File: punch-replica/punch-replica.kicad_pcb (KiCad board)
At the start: 2 copper layers, 90 x 80 mm, 67 parts, among them J10 Screw_Terminal_01x03, J11 Screw_Terminal_01x03, J12 Screw_Terminal_01x02, J2 12V PSU, J3 5V OUT, J4 5V OUT, J5 LOAD CELL, J6 COIN SLOT, J7 Conn_01x02_Socket, J9 IDC_Connector, K1 SRD-05VDC-SL-C, K2 SRD-05VDC-SL-C, Q1 BSS138, Q2 BSS138, Q3 Q_NMOS_Depletion_GSD, Q4 Q_NMOS_Depletion_GSD, SW1 SW_Push, SW2 SW_Push, U1 LM2596S-5, U2 AMS1117-3.3, U3 CH340C, U4 PC817, U5 PC817, U6 ESP32-WROOM-32, U7 DFR0299

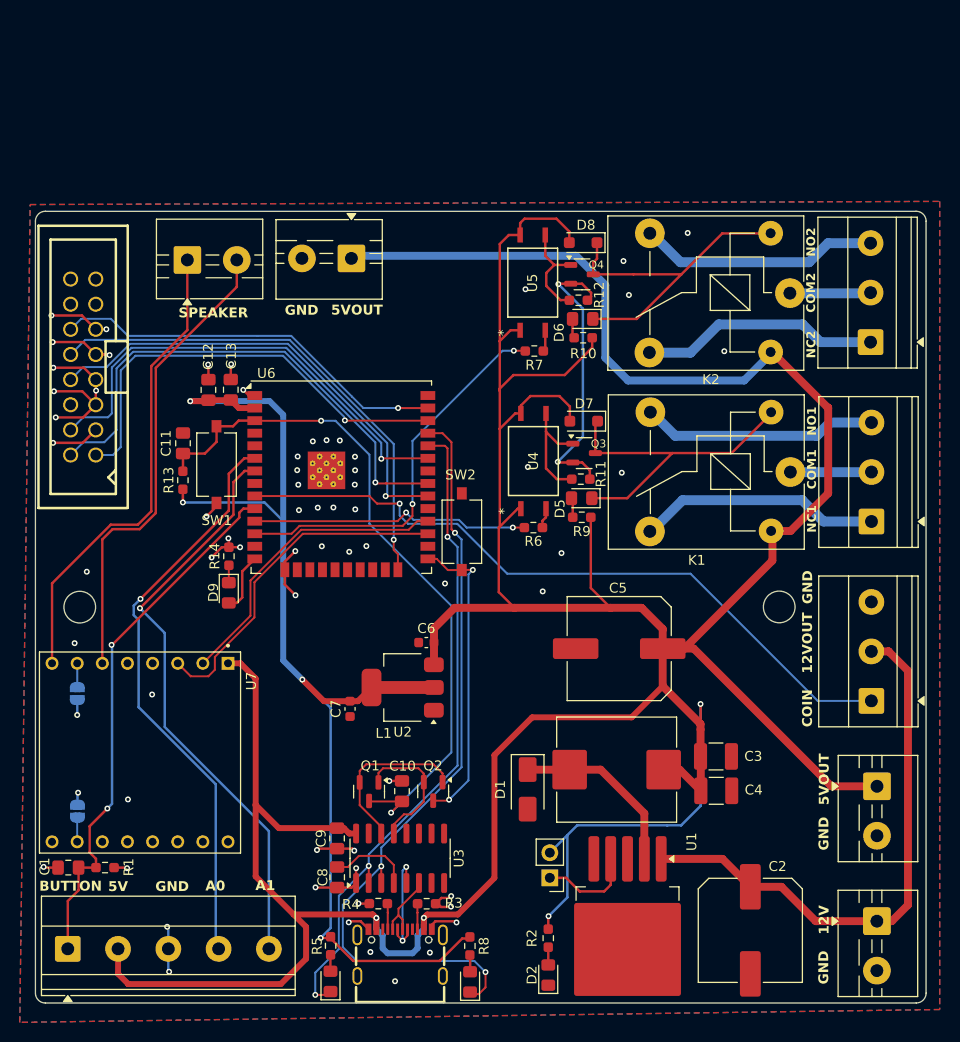
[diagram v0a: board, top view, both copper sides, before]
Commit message: - adjustment
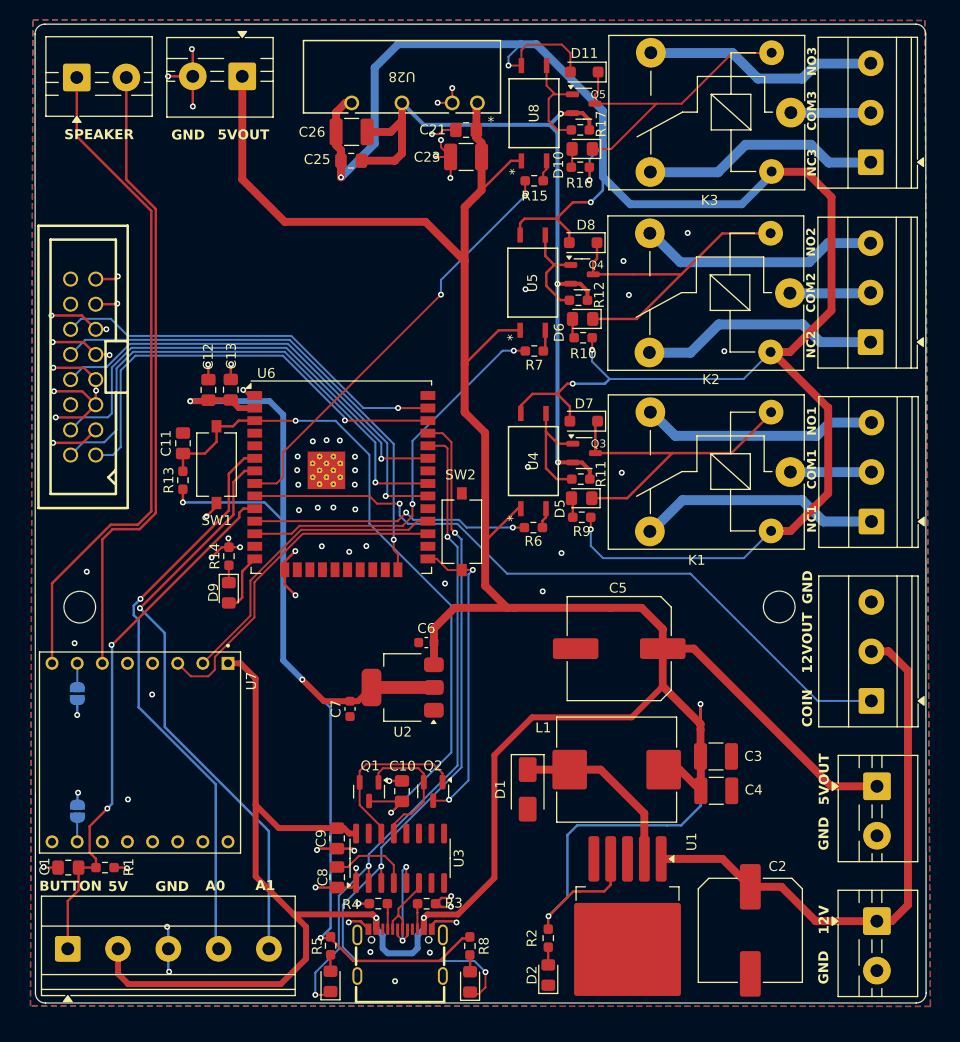
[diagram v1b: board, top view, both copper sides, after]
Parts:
- removed J7: Conn_01x02_Socket, Connector_PinHeader_2.54mm:PinHeader_1x02_P2.54mm_Vertical
- added C21: 10uF, Capacitor_SMD:C_0805_2012Metric_Pad1.18x1.45mm_HandSolder, F.Cu at (207.3, 59.9)
- added C23: 100uF, Capacitor_SMD:C_1210_3225Metric_Pad1.33x2.70mm_HandSolder, F.Cu at (207.3, 62.6)
- added C25: 10uF, Capacitor_SMD:C_0805_2012Metric_Pad1.18x1.45mm_HandSolder, F.Cu at (195.7, 63.0)
- added C26: 100uF, Capacitor_SMD:C_1210_3225Metric_Pad1.33x2.70mm_HandSolder, F.Cu at (195.7, 60.0)
- added D10: LED, LED_SMD:LED_0805_2012Metric_Pad1.15x1.40mm_HandSolder, F.Cu at (219.0, 61.8)
- added D11: 1N4001, Diode_SMD:D_SOD-123F, F.Cu at (219.2, 54.0)
- added J1: Screw_Terminal_01x03, TerminalBlock_Phoenix:TerminalBlock_Phoenix_MKDS-1,5-3_1x03_P5.00mm_Horizontal, F.Cu at (248.2, 63.1)
- added K3: SRD-05VDC-SL-C, Relay_THT:Relay_SPDT_SANYOU_SRD_Series_Form_C, F.Cu at (240.1, 58.1)
- added Q5: Q_NMOS_Depletion_GSD, Package_TO_SOT_SMD:SOT-23-3, F.Cu at (219.2, 57.2)
- added R15: 470, Resistor_SMD:R_0603_1608Metric_Pad0.98x0.95mm_HandSolder, F.Cu at (214.2, 65.0)
- added R16: 1k, Resistor_SMD:R_0603_1608Metric_Pad0.98x0.95mm_HandSolder, F.Cu at (218.8, 63.6)
- added R17: 10K, Resistor_SMD:R_0603_1608Metric_Pad0.98x0.95mm_HandSolder, F.Cu at (218.8, 59.8)
- added U28: B0505S-2WR3, Library:B_S-2WR2_MNS, F.Cu at (208.4, 57.1)
- added U8: PC817, Library:APC-817xx-SL_AMB, F.Cu at (214.1, 58.1)
- moved J12 21.6 mm to (167.9, 54.5)
- moved J4 21.5 mm to (184.7, 54.4)
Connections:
- D7 pad 2: +5V -> +5VA
- D8 pad 2: +5V -> +5VA
- K1 pad 5: +5V -> +5VA
- K2 pad 5: +5V -> +5VA
- R10 pad 1: +5V -> +5VA
- R9 pad 1: +5V -> +5VA
- U1 pad 4: Net-(J7-Pin_1) -> +5V
- U4 pad 4: +5V -> +5VA
- U5 pad 4: +5V -> +5VA
- U6 pad 8: unconnected-(U6-IO32-Pad8) -> DC_DRV_3
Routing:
- net +5VA: track 0.00 -> 218.0 mm, vias 0 -> 7
- net +5V: track 431.4 -> 364.7 mm
- net GNDPWR: track 29.1 -> 78.3 mm, vias 2 -> 3
- net DC_DRV_3: track 0.00 -> 43.2 mm, vias 0 -> 2
- net Net-(D10-K): track 0.00 -> 31.7 mm
- net GND: track 81.2 -> 105.5 mm, vias 67 -> 78
- net NC3: track 0.00 -> 24.2 mm
- net NO3: track 0.00 -> 23.9 mm
- net Net-(J12-Pin_1): track 48.0 -> 68.1 mm
- net Net-(J12-Pin_2): track 48.0 -> 64.3 mm
- net Net-(Q5-G): track 0.00 -> 10.8 mm
- net Net-(J7-Pin_1): track 9.62 -> 0.00 mm
- net COM3: track 0.00 -> 8.09 mm
- net Net-(R15-Pad2): track 0.00 -> 2.16 mm
- net Net-(D10-A): track 0.00 -> 1.89 mm
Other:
- board size 90 x 80 mm -> 90 x 98.9 mm
- board text added: "COM3"
- board text added: "NC3"
- board text added: "NO3"
